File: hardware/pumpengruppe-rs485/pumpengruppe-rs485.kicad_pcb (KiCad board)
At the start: 2 copper layers, 160 x 110 mm, 25 parts, among them J1 RJ45_IN, J2 RJ45_OUT, J3 RS485_IN, J4 RS485_OUT, K1 PUMP_RELAY, K2 OPEN_RELAY, K3 CLOSE_RELAY, U1 ESP32-WROOM-32U, U2 MAX31865_VL, U3 MAX31865_RL, U4 ISO_RS485, U5 3V3_REG, U6 CP2102N_USB_UART, X1 230V_IN, X2 PUMPE, X3 MISCHER, X4 RTD_VL, X5 RTD_RL, X6 USB_C_SERVICE_FLASH

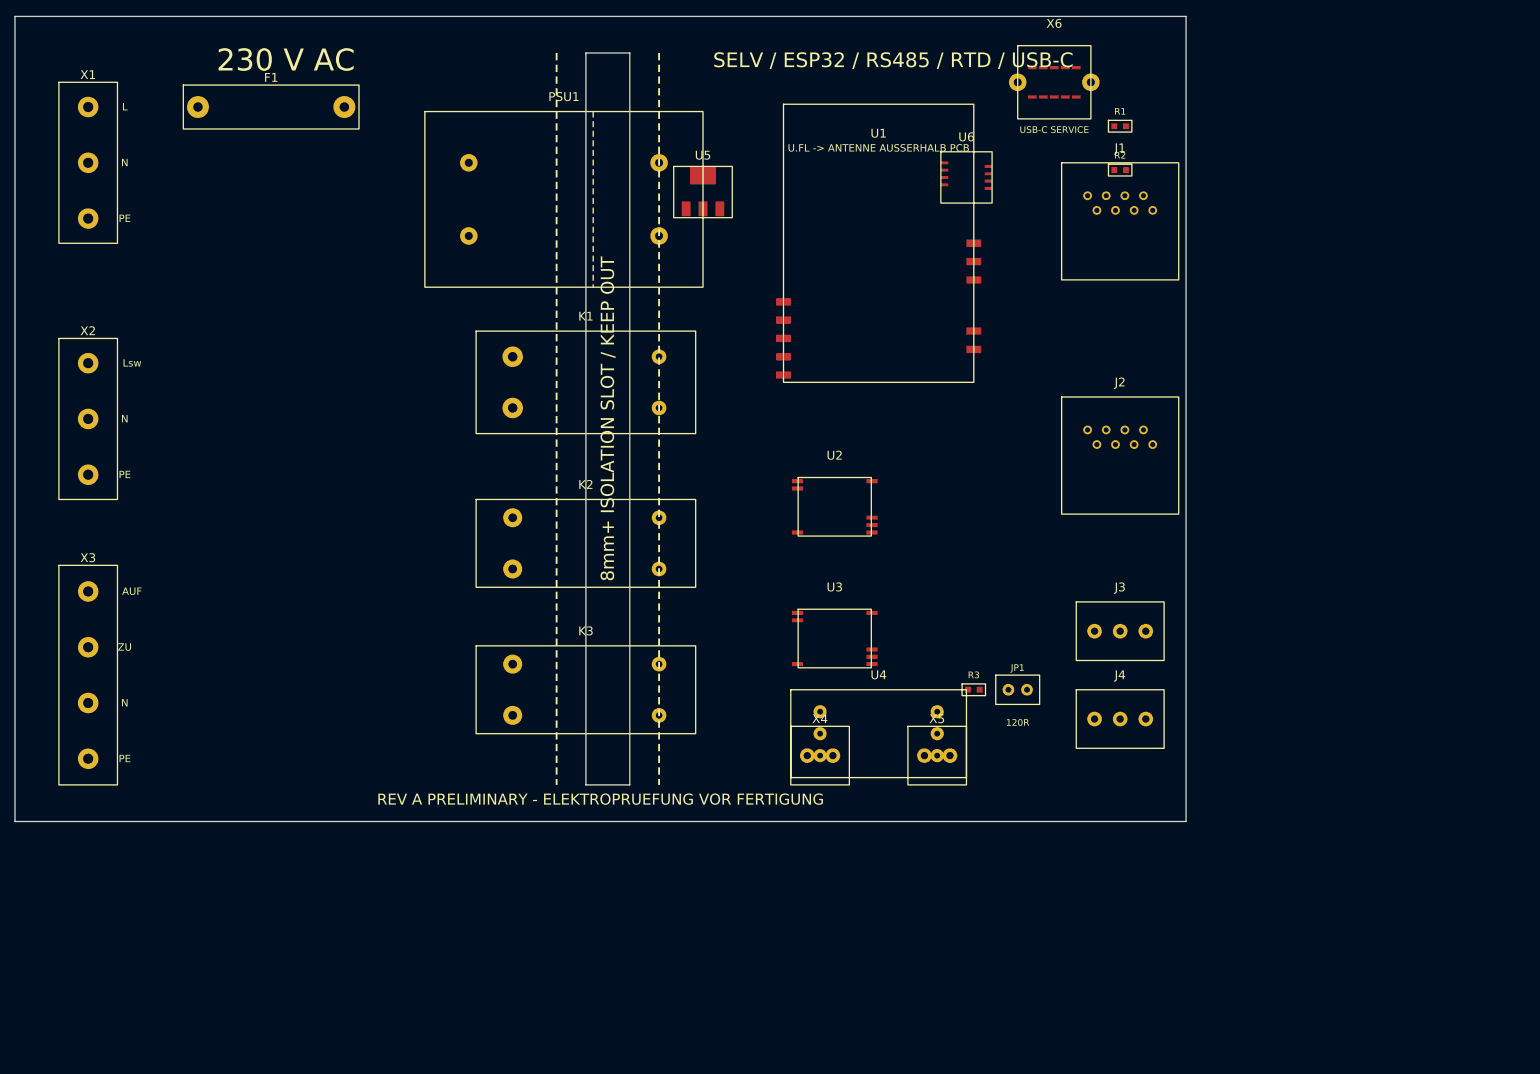
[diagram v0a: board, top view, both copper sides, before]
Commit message: sicherung
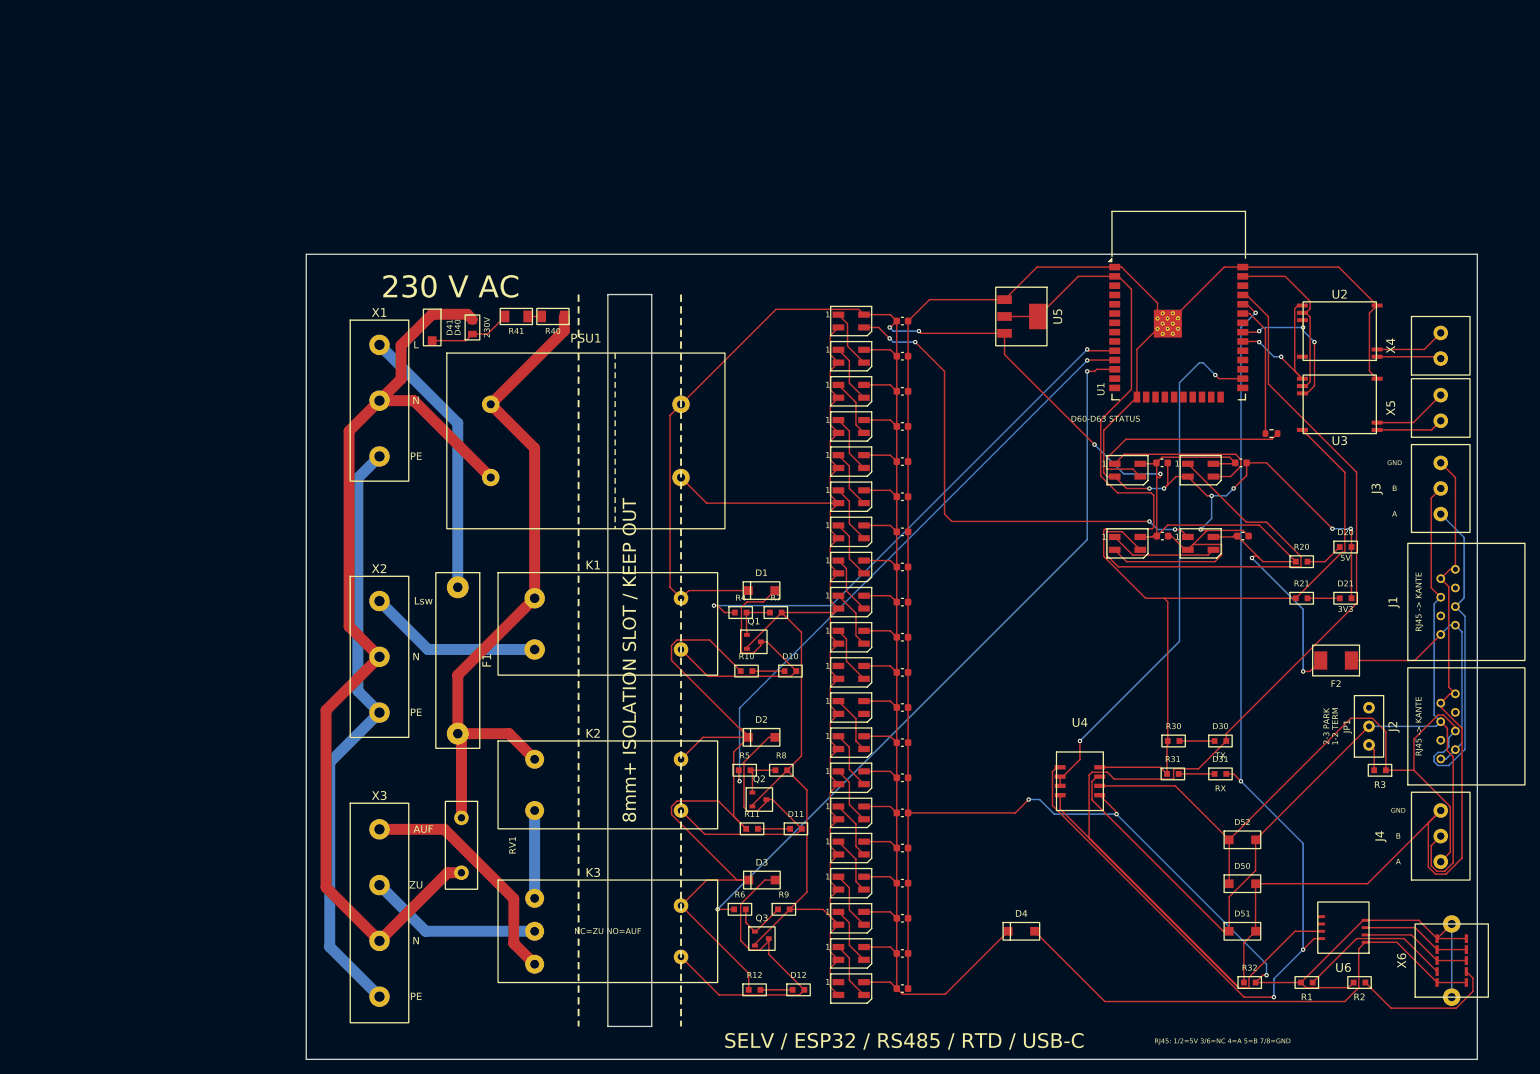
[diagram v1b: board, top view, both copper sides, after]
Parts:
- added C60: 100n_RGB_LED, Capacitor_SMD:C_0603_1608Metric, F.Cu at (156.8, 71.0)
- added C61: 100n_RGB_LED, Capacitor_SMD:C_0603_1608Metric, F.Cu at (167.8, 71.0)
- added C62: 100n_RGB_LED, Capacitor_SMD:C_0603_1608Metric, F.Cu at (156.7, 61.0)
- added C63: 100n_RGB_LED, Capacitor_SMD:C_0603_1608Metric, F.Cu at (167.5, 61.0)
- added C64: 100n_RGB_LED, Capacitor_SMD:C_0603_1608Metric, F.Cu at (121.2, 41.6)
- added C65: 100n_RGB_LED, Capacitor_SMD:C_0603_1608Metric, F.Cu at (121.2, 46.4)
- added C66: 100n_RGB_LED, Capacitor_SMD:C_0603_1608Metric, F.Cu at (121.2, 51.2)
- added C67: 100n_RGB_LED, Capacitor_SMD:C_0603_1608Metric, F.Cu at (121.2, 56.0)
- added C68: 100n_RGB_LED, Capacitor_SMD:C_0603_1608Metric, F.Cu at (121.2, 60.8)
- added C69: 100n_RGB_LED, Capacitor_SMD:C_0603_1608Metric, F.Cu at (121.2, 65.6)
- added C70: 100n_RGB_LED, Capacitor_SMD:C_0603_1608Metric, F.Cu at (121.2, 70.4)
- added C71: 100n_RGB_LED, Capacitor_SMD:C_0603_1608Metric, F.Cu at (121.2, 75.2)
- added C72: 100n_RGB_LED, Capacitor_SMD:C_0603_1608Metric, F.Cu at (121.2, 80.0)
- added C73: 100n_RGB_LED, Capacitor_SMD:C_0603_1608Metric, F.Cu at (121.2, 84.8)
- added C74: 100n_RGB_LED, Capacitor_SMD:C_0603_1608Metric, F.Cu at (121.2, 89.6)
- added C75: 100n_RGB_LED, Capacitor_SMD:C_0603_1608Metric, F.Cu at (121.2, 94.4)
- added C76: 100n_RGB_LED, Capacitor_SMD:C_0603_1608Metric, F.Cu at (121.2, 99.2)
- added C77: 100n_RGB_LED, Capacitor_SMD:C_0603_1608Metric, F.Cu at (121.2, 104.0)
- added C78: 100n_RGB_LED, Capacitor_SMD:C_0603_1608Metric, F.Cu at (121.2, 108.8)
- added C79: 100n_RGB_LED, Capacitor_SMD:C_0603_1608Metric, F.Cu at (121.2, 113.6)
- added C80: 100n_RGB_LED, Capacitor_SMD:C_0603_1608Metric, F.Cu at (121.2, 118.4)
- added C81: 100n_RGB_LED, Capacitor_SMD:C_0603_1608Metric, F.Cu at (121.2, 123.2)
- added C82: 100n_RGB_LED, Capacitor_SMD:C_0603_1608Metric, F.Cu at (121.2, 128.0)
- added C83: 100n_RGB_LED, Capacitor_SMD:C_0603_1608Metric, F.Cu at (121.2, 132.8)
- added D1: SS14_FLYBACK_PUMP, FW_Pumpengruppe:D_SOD123, F.Cu at (102.0, 78.5)
- added D10: LED_PUMP, FW_Pumpengruppe:LED_0603, F.Cu at (106.0, 89.5)
- added D11: LED_MIX_ENABLE, FW_Pumpengruppe:LED_0603, F.Cu at (106.7, 111.0)
- added D12: LED_MIX_DIR, FW_Pumpengruppe:LED_0603, F.Cu at (107.0, 133.0)
- added D2: SS14_FLYBACK_MIX_ENABLE, FW_Pumpengruppe:D_SOD123, F.Cu at (102.0, 98.5)
- added D20: LED_5V, FW_Pumpengruppe:LED_0603, F.Cu at (181.8, 72.5)
- added D21: LED_3V3, FW_Pumpengruppe:LED_0603, F.Cu at (181.8, 79.5)
- added D3: SS14_FLYBACK_MIX_DIR, FW_Pumpengruppe:D_SOD123, F.Cu at (102.0, 118.0)
- added D30: LED_RS485_TX, FW_Pumpengruppe:LED_0603, F.Cu at (164.7, 99.0)
- added D31: LED_RS485_RX, FW_Pumpengruppe:LED_0603, F.Cu at (164.7, 103.5)
- added D4: SS14_USB_TO_5V, FW_Pumpengruppe:D_SOD123, F.Cu at (137.5, 125.0)
- added D40: LED_230VAC, LED_SMD:LED_0805_2012Metric, F.Cu at (62.5, 42.5)
- added D41: 1N4148_ANTI_PARALLEL, Diode_SMD:D_SOD-123, F.Cu at (57.0, 42.5)
- added D50: TVS_RS485_A_COM, Diode_SMD:D_SOD-123, F.Cu at (167.7, 118.5)
- added D51: TVS_RS485_B_COM, Diode_SMD:D_SOD-123, F.Cu at (167.7, 125.0)
- added D52: TVS_RS485_A_B, Diode_SMD:D_SOD-123, F.Cu at (167.7, 112.5)
- added D60: SK6812MINI_STATUS_1, LED_SMD:LED_SK6812MINI_PLCC4_3.5x3.5mm_P1.75mm, F.Cu at (152.0, 62.0)
- added D61: SK6812MINI_STATUS_2, LED_SMD:LED_SK6812MINI_PLCC4_3.5x3.5mm_P1.75mm, F.Cu at (162.0, 62.0)
- added D62: SK6812MINI_STATUS_3, LED_SMD:LED_SK6812MINI_PLCC4_3.5x3.5mm_P1.75mm, F.Cu at (152.0, 72.0)
- added D63: SK6812MINI_STATUS_4, LED_SMD:LED_SK6812MINI_PLCC4_3.5x3.5mm_P1.75mm, F.Cu at (162.0, 72.0)
- added D64: SK6812MINI_VALVE_5PCT, LED_SMD:LED_SK6812MINI_PLCC4_3.5x3.5mm_P1.75mm, F.Cu at (114.2, 41.6)
- added D65: SK6812MINI_VALVE_10PCT, LED_SMD:LED_SK6812MINI_PLCC4_3.5x3.5mm_P1.75mm, F.Cu at (114.2, 46.4)
- added D66: SK6812MINI_VALVE_15PCT, LED_SMD:LED_SK6812MINI_PLCC4_3.5x3.5mm_P1.75mm, F.Cu at (114.2, 51.2)
- added D67: SK6812MINI_VALVE_20PCT, LED_SMD:LED_SK6812MINI_PLCC4_3.5x3.5mm_P1.75mm, F.Cu at (114.2, 56.0)
- added D68: SK6812MINI_VALVE_25PCT, LED_SMD:LED_SK6812MINI_PLCC4_3.5x3.5mm_P1.75mm, F.Cu at (114.2, 60.8)
- added D69: SK6812MINI_VALVE_30PCT, LED_SMD:LED_SK6812MINI_PLCC4_3.5x3.5mm_P1.75mm, F.Cu at (114.2, 65.6)
- added D70: SK6812MINI_VALVE_35PCT, LED_SMD:LED_SK6812MINI_PLCC4_3.5x3.5mm_P1.75mm, F.Cu at (114.2, 70.4)
- added D71: SK6812MINI_VALVE_40PCT, LED_SMD:LED_SK6812MINI_PLCC4_3.5x3.5mm_P1.75mm, F.Cu at (114.2, 75.2)
- added D72: SK6812MINI_VALVE_45PCT, LED_SMD:LED_SK6812MINI_PLCC4_3.5x3.5mm_P1.75mm, F.Cu at (114.2, 80.0)
- added D73: SK6812MINI_VALVE_50PCT, LED_SMD:LED_SK6812MINI_PLCC4_3.5x3.5mm_P1.75mm, F.Cu at (114.2, 84.8)
- added D74: SK6812MINI_VALVE_55PCT, LED_SMD:LED_SK6812MINI_PLCC4_3.5x3.5mm_P1.75mm, F.Cu at (114.2, 89.6)
- added D75: SK6812MINI_VALVE_60PCT, LED_SMD:LED_SK6812MINI_PLCC4_3.5x3.5mm_P1.75mm, F.Cu at (114.2, 94.4)
- added D76: SK6812MINI_VALVE_65PCT, LED_SMD:LED_SK6812MINI_PLCC4_3.5x3.5mm_P1.75mm, F.Cu at (114.2, 99.2)
- added D77: SK6812MINI_VALVE_70PCT, LED_SMD:LED_SK6812MINI_PLCC4_3.5x3.5mm_P1.75mm, F.Cu at (114.2, 104.0)
- added D78: SK6812MINI_VALVE_75PCT, LED_SMD:LED_SK6812MINI_PLCC4_3.5x3.5mm_P1.75mm, F.Cu at (114.2, 108.8)
- added D79: SK6812MINI_VALVE_80PCT, LED_SMD:LED_SK6812MINI_PLCC4_3.5x3.5mm_P1.75mm, F.Cu at (114.2, 113.6)
- added D80: SK6812MINI_VALVE_85PCT, LED_SMD:LED_SK6812MINI_PLCC4_3.5x3.5mm_P1.75mm, F.Cu at (114.2, 118.4)
- added D81: SK6812MINI_VALVE_90PCT, LED_SMD:LED_SK6812MINI_PLCC4_3.5x3.5mm_P1.75mm, F.Cu at (114.2, 123.2)
- added D82: SK6812MINI_VALVE_95PCT, LED_SMD:LED_SK6812MINI_PLCC4_3.5x3.5mm_P1.75mm, F.Cu at (114.2, 128.0)
- added D83: SK6812MINI_VALVE_100PCT, LED_SMD:LED_SK6812MINI_PLCC4_3.5x3.5mm_P1.75mm, F.Cu at (114.2, 132.8)
- added F2: PTC_BUS_5V, Fuse:Fuse_1812_4532Metric, F.Cu at (180.5, 88.0)
- added Q1: AO3400A_PUMP, FW_Pumpengruppe:SOT23_NMOS, F.Cu at (101.0, 85.5)
- added Q2: AO3400A_MIX_ENABLE, FW_Pumpengruppe:SOT23_NMOS, F.Cu at (101.7, 107.0)
- added Q3: AO3400A_MIX_DIR, FW_Pumpengruppe:SOT23_NMOS, F.Cu at (102.0, 126.0)
- added R10: 2k2_LED_PUMP, FW_Pumpengruppe:R_0603, F.Cu at (100.0, 89.5)
- added R11: 2k2_LED_MIX_ENABLE, FW_Pumpengruppe:R_0603, F.Cu at (100.7, 111.0)
- added R12: 2k2_LED_MIX_DIR, FW_Pumpengruppe:R_0603, F.Cu at (101.0, 133.0)
- added R20: 2k2_LED_5V, FW_Pumpengruppe:R_0603, F.Cu at (175.8, 74.5)
- added R21: 1k5_LED_3V3, FW_Pumpengruppe:R_0603, F.Cu at (175.8, 79.5)
- added R30: 4k7_LED_TX, FW_Pumpengruppe:R_0603, F.Cu at (158.3, 99.0)
- added R31: 4k7_LED_RX, FW_Pumpengruppe:R_0603, F.Cu at (158.2, 103.5)
- added R32: 0R_BUS_0V_LINK, FW_Pumpengruppe:R_0603, F.Cu at (168.7, 132.0)
- added R4: 100R_GATE_PUMP, FW_Pumpengruppe:R_0603, F.Cu at (99.2, 81.5)
- added R40: 150k_LED_230V_1, Resistor_SMD:R_1206_3216Metric, F.Cu at (73.5, 41.0)
- added R41: 150k_LED_230V_2, Resistor_SMD:R_1206_3216Metric, F.Cu at (68.5, 41.0)
- added R5: 100R_GATE_MIX_ENABLE, FW_Pumpengruppe:R_0603, F.Cu at (99.7, 103.0)
- added R6: 100R_GATE_MIX_DIR, FW_Pumpengruppe:R_0603, F.Cu at (99.0, 122.0)
- added R60: 330R_RGB_DATA, Resistor_SMD:R_0603_1608Metric, F.Cu at (171.7, 57.0)
- added R7: 100k_GATE_PD, FW_Pumpengruppe:R_0603, F.Cu at (104.0, 81.5)
- added R8: 100k_GATE_PD, FW_Pumpengruppe:R_0603, F.Cu at (104.7, 103.0)
- added R9: 100k_GATE_PD, FW_Pumpengruppe:R_0603, F.Cu at (105.0, 122.0)
- added RV1: MOV_275VAC, Varistor:RV_Disc_D12mm_W3.9mm_P7.5mm, F.Cu at (61.0, 113.2)
- J1, J2: footprint FW_Pumpengruppe:RJ45_SHIELDED_GENERIC -> Connector_RJ:RJ45_Amphenol_54602-x08_Horizontal
- JP1: value RS485_TERM_ON -> RS485_TERM_ON_PARK; footprint FW_Pumpengruppe:JP_2_254 -> Connector_PinHeader_2.54mm:PinHeader_1x03_P2.54mm_Vertical
- K2: value OPEN_RELAY -> MIX_ENABLE_RELAY
- K3: value CLOSE_RELAY -> MIX_DIR_SPDT_RELAY; footprint FW_Pumpengruppe:Relay_SPST_8A -> FW_Pumpengruppe:Relay_SPDT_8A
- PSU1: value IRM-05-5 -> HLK-5M05; footprint FW_Pumpengruppe:ACDC_IRM05 -> Converter_ACDC:Converter_ACDC_Hi-Link_HLK-5Mxx
- U1: value ESP32-WROOM-32U -> ESP32-WROOM-32D; footprint FW_Pumpengruppe:ESP32_WROOM_KEEP_OUT -> RF_Module:ESP32-WROOM-32D
- U4: value ISO_RS485 -> MAX3485_SOIC8; footprint FW_Pumpengruppe:ISO_RS485_MODULE -> Package_SO:SOIC-8_3.9x4.9mm_P1.27mm
- X6: footprint FW_Pumpengruppe:USB_C_SERVICE -> Connector_USB:USB_C_Receptacle_HRO_TYPE-C-31-M-12
- moved X6 131.7 mm to (196.3, 129.0), turned to 90 degrees
- moved R1 119.7 mm to (176.5, 132.0), turned to 180 degrees
- moved R2 115.7 mm to (183.7, 132.0), turned to 180 degrees
- moved U6 114.7 mm to (181.5, 124.5), turned to 180 degrees
- moved X4 101.6 mm to (194.8, 45.0), turned to 90 degrees
- moved X5 83.6 mm to (194.8, 53.5), turned to 90 degrees
- moved F1 79.8 mm to (60.5, 88.0), turned to -90 degrees
- moved U3 76.1 mm to (181.0, 53.0), turned to 180 degrees
- moved U2 73.1 mm to (181.0, 43.0), turned to 180 degrees
- moved J1 70.3 mm to (198.3, 80.0), turned to 90 degrees
- moved J2 60.1 mm to (198.3, 97.0), turned to 90 degrees
- moved R3 56.6 mm to (186.5, 103.0), turned to 180 degrees
- moved X1 51.4 mm to (49.8, 52.5)
- moved X2 51.4 mm to (49.8, 87.5)
- moved X3 51.4 mm to (49.8, 122.5)
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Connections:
- J1 pad 1: (no net) -> BUS_5V
- J1 pad 2: (no net) -> BUS_5V
- J2 pad 1: (no net) -> BUS_5V
- J2 pad 2: (no net) -> BUS_5V
- K1 pad A2: PUMP_DRV -> PUMP_COIL_L
- K2 pad 2: L_OPEN -> MIX_L_EN
- K2 pad A2: OPEN_DRV -> MIX_ENABLE_COIL_L
- K3 pad A2: CLOSE_DRV -> MIX_DIR_COIL_L
- U1 pad 1: +3V3 -> GND
- U1 pad 10: UART_RX -> PUMP_DRV
- U1 pad 2: GND -> +3V3
- U1 pad 3: PUMP_DRV -> (no net)
- U1 pad 4: OPEN_DRV -> (no net)
- U1 pad 5: CLOSE_DRV -> (no net)
- U1 pad 6: SPI_MOSI -> (no net)
- U1 pad 7: SPI_MISO -> (no net)
- U1 pad 8: SPI_SCK -> (no net)
- U1 pad 9: UART_TX -> (no net)
- U4 pad 1: +5V -> UART_RX
- U4 pad 2: UART_TX -> RS485_DE
- U4 pad 3: UART_RX -> RS485_DE
- U4 pad 4: RS485_A -> UART_TX
- U4 pad 5: RS485_B -> GND
- U4 pad 6: RS485_GND -> RS485_A
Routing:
- net GND: track 0.00 -> 628.2 mm, vias 0 -> 10
- net +5V: track 0.00 -> 519.0 mm, vias 0 -> 6
- net UART_TX: track 0.00 -> 186.6 mm
- net +3V3: track 0.00 -> 161.7 mm
- net UART_RX: track 0.00 -> 154.3 mm, vias 0 -> 4
- net N: track 0.00 -> 138.9 mm
- net RS485_A: track 0.00 -> 138.1 mm
- net RS485_B: track 0.00 -> 138.0 mm
- net RS485_GND: track 0.00 -> 117.3 mm
- net MIX_DIR_DRV: track 0.00 -> 100.5 mm, vias 0 -> 2
- net L_FUSED: track 0.00 -> 91.7 mm
- net MIX_ENABLE_DRV: track 0.00 -> 82.5 mm, vias 0 -> 2
- net PE: track 0.00 -> 81.9 mm
- net RS485_DE: track 0.00 -> 72.7 mm, vias 0 -> 2
- net PUMP_DRV: track 0.00 -> 72.6 mm, vias 0 -> 2
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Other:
- outline, holes or cut-outs redrawn
- board text added: "A"
- board text added: "B"
- board text added: "D60-D63 STATUS"
- board text added: "GND"
- board text added: "RJ45: 1/2=5V 3/6=NC 4=A 5=B 7/8=GND"
- board text removed: "REV A PRELIMINARY - ELEKTROPRUEFUNG VOR FERTIGUNG"
